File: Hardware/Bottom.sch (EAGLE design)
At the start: 106 parts, among them IC1 OP491SOIC_N14, IC2 74AC74D, IC3 74LVC1G17DCK, IC4 LT6231, IC5 SN74CBT3253SOIC16, Q1 DMPH6050SK3, Q2 25MHz

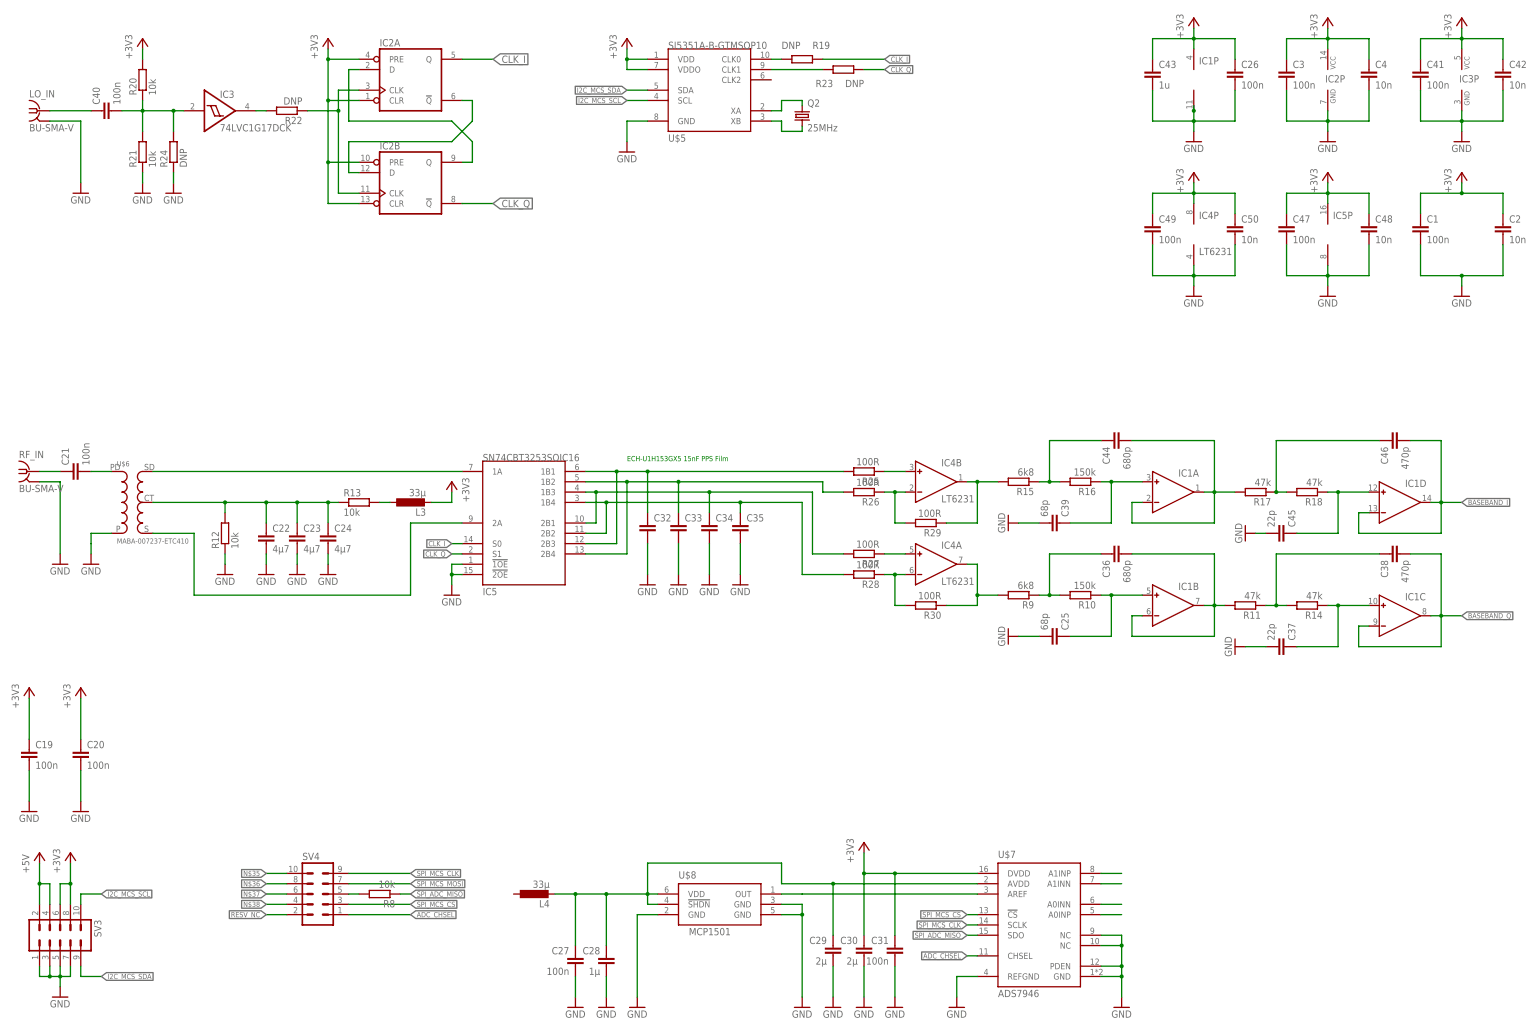
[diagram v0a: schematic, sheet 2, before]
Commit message: Add various parts
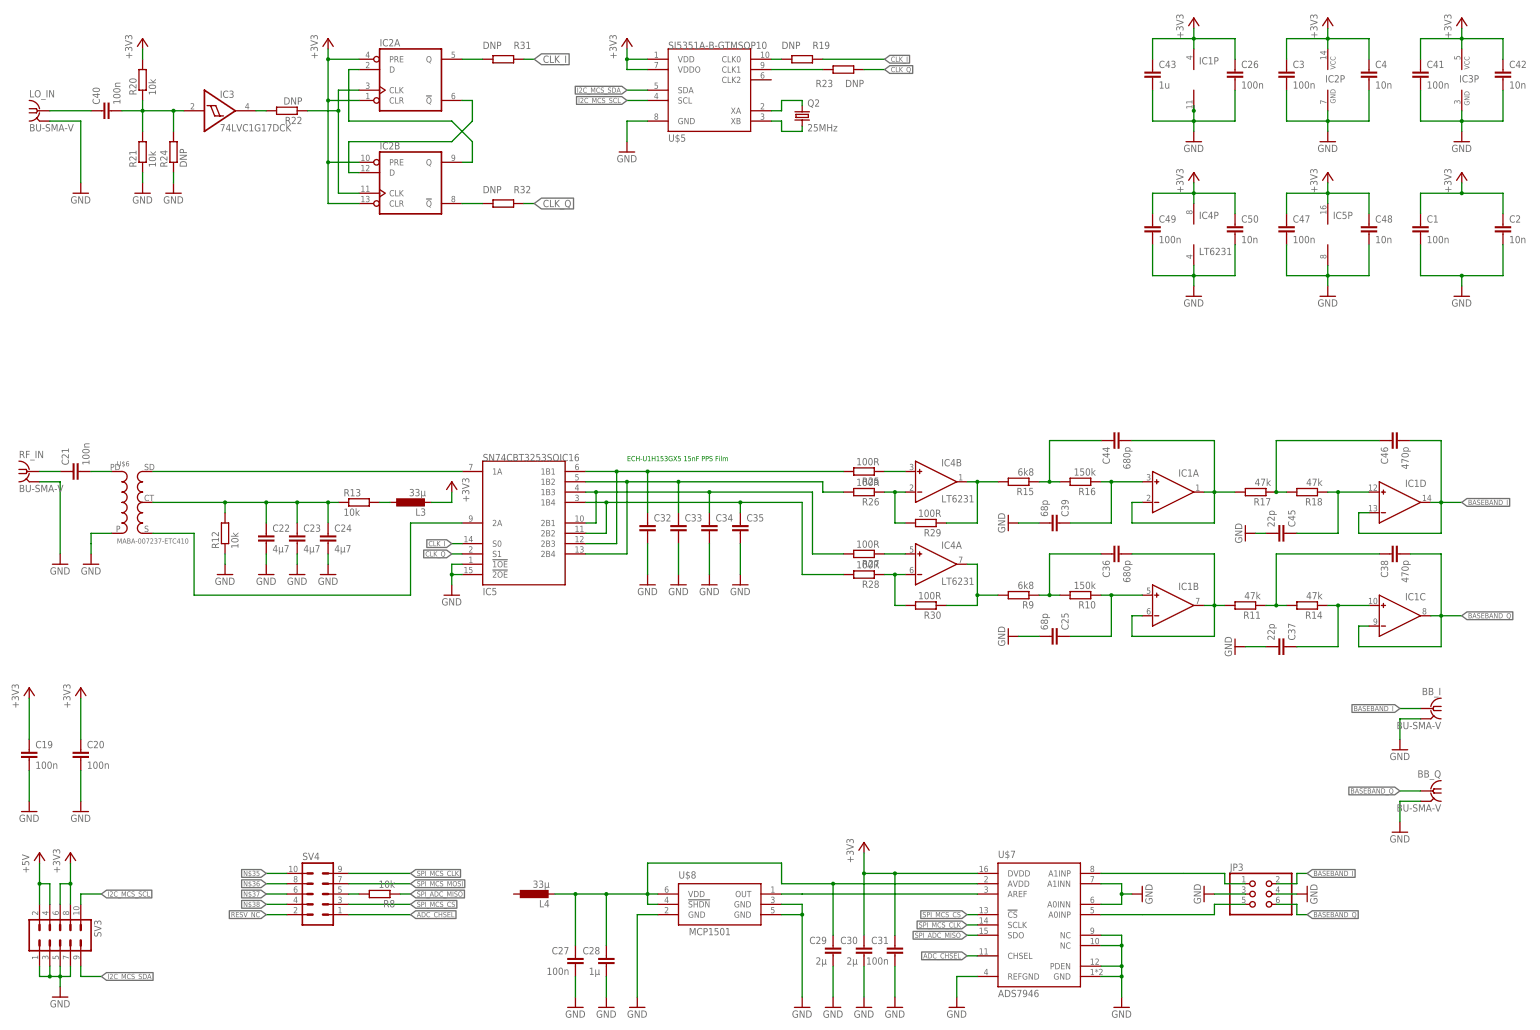
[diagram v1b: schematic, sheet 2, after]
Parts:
- added BB_I, BB_Q: BU-SMA-V, con-coax:BU-SMA-V
- added JP3: (no value), pinhead:PINHD-2X3
- added R31, R32: DNP, rcl:R-EU_R0603
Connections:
- removed net N$25: U$7.A1INP
- removed net N$28: U$7.A0INN
- new net N$58: IC2B.!Q, R32.2
- new net N$59: IC2A.Q, R31.2
- net BASEBAND_I: now also BB_I.1, JP3.2
- net BASEBAND_Q: now also BB_Q.1, JP3.6
- net CLK_I: now also R31.1; no longer IC2A.Q
- net CLK_Q: now also R32.1; no longer IC2B.!Q
- net GND: now also BB_I.2, BB_Q.2, JP3.3, JP3.4, U$7.A0INN, U$7.A1INN
- net N$26: now also JP3.1, U$7.A1INP; no longer U$7.A1INN
- net N$32: now also JP3.5

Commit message: Add various parts
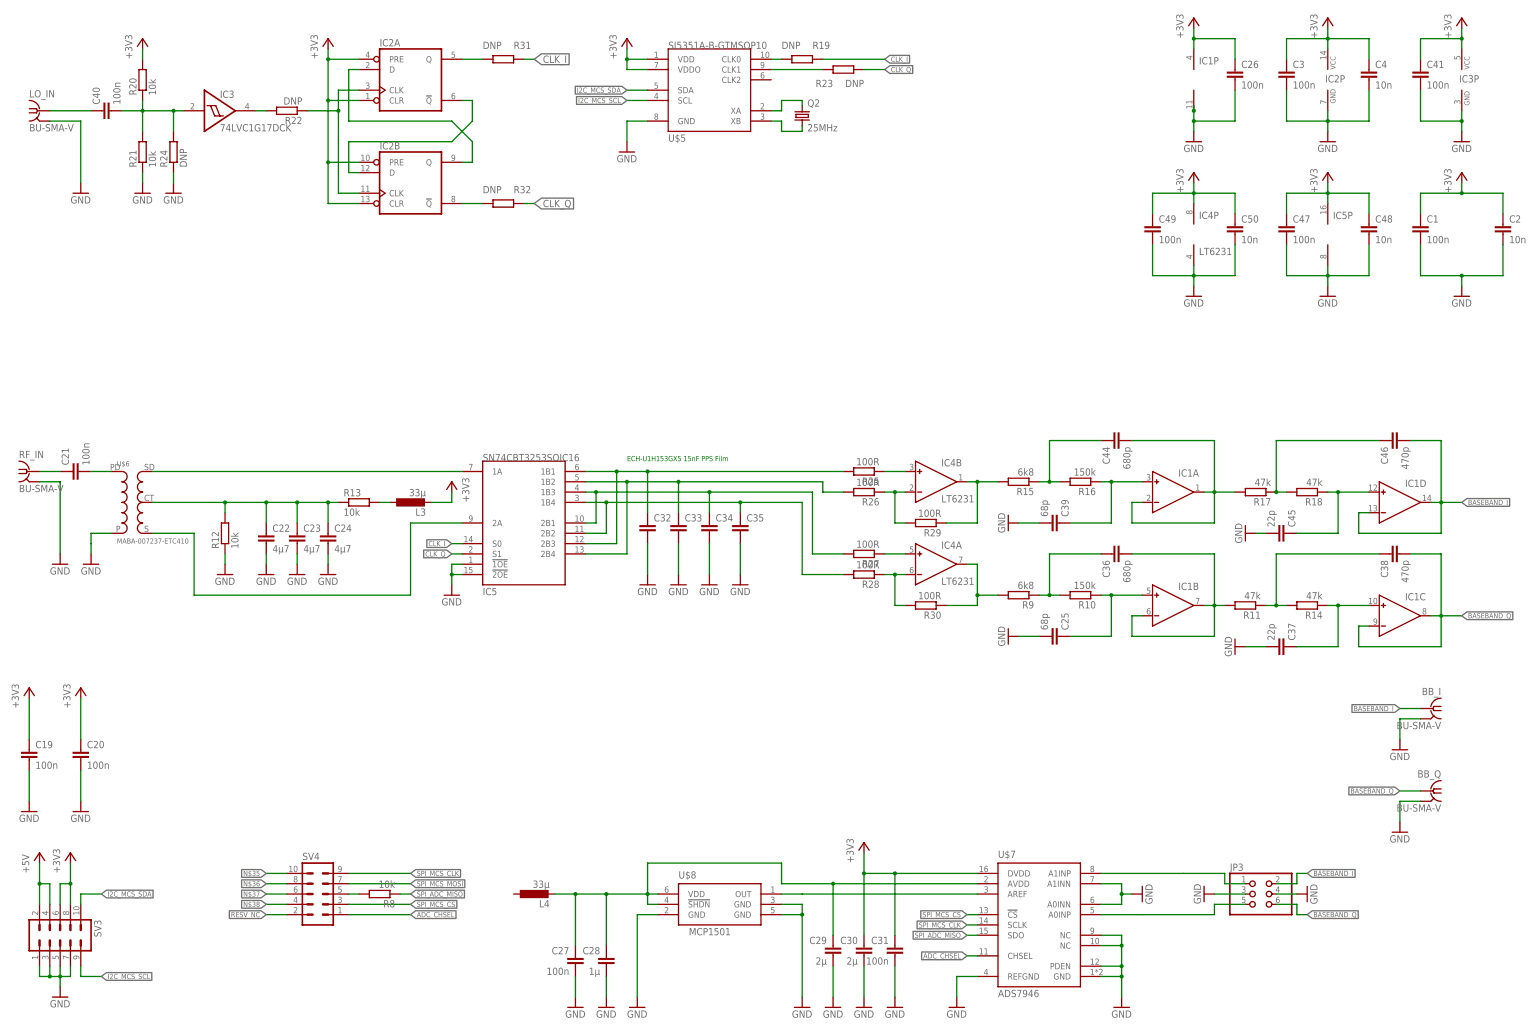
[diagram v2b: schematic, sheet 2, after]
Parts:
- removed C42: 10n, rcl:C-EUC0402
- removed C43: 1u, rcl:C-EUC0603
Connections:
- net +3V3: no longer C42.1, C43.1
- net GND: no longer C42.2, C43.2
- net I2C_MCS_SCL: now also SV3.9; no longer SV3.10
- net I2C_MCS_SDA: now also SV3.10; no longer SV3.9
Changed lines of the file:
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@@
 <part name="+3V11" library="supply1" library_urn="urn:adsk.eagle:library:371" deviceset="+3V3" device=""/>
 <part name="C41" library="rcl" library_urn="urn:adsk.eagle:library:334" deviceset="C-EU" device="C0402" package3d_urn="urn:adsk.eagle:package:23626/1" value="100n"/>
-<part name="C42" library="rcl" library_urn="urn:adsk.eagle:library:334" deviceset="C-EU" device="C0402" package3d_urn="urn:adsk.eagle:package:23626/1" value="10n"/>
 <part name="GND55" library="supply1" library_urn="urn:adsk.eagle:library:371" deviceset="GND" device=""/>
 <part name="+3V12" library="supply1" library_urn="urn:adsk.eagle:library:371" deviceset="+3V3" device=""/>
-<part name="C43" library="rcl" library_urn="urn:adsk.eagle:library:334" deviceset="C-EU" device="C0603" package3d_urn="urn:adsk.eagle:package:23616/2" value="1u"/>
 <part name="RF_IN" library="con-coax" library_urn="urn:adsk.eagle:library:133" deviceset="BU-SMA-V" device="" package3d_urn="urn:adsk.eagle:package:6211/1"/>
 <part name="LO_IN" library="con-coax" library_urn="urn:adsk.eagle:library:133" deviceset="BU-SMA-V" device="" package3d_urn="urn:adsk.eagle:package:6211/1"/>
@@
 <attribute name="VALUE" x="359.664" y="236.601" size="1.778" layer="96"/>
 </instance>
-<instance part="C42" gate="G$1" x="378.46" y="241.3" smashed="yes">
-<attribute name="NAME" x="379.984" y="241.681" size="1.778" layer="95"/>
-<attribute name="VALUE" x="379.984" y="236.601" size="1.778" layer="96"/>
-</instance>
 <instance part="GND55" gate="1" x="368.3" y="223.52" smashed="yes">
 <attribute name="VALUE" x="365.76" y="220.98" size="1.778" layer="96"/>
@@
 <instance part="+3V12" gate="G$1" x="368.3" y="254" smashed="yes">
 <attribute name="VALUE" x="365.76" y="248.92" size="1.778" layer="96" rot="R90"/>
-</instance>
-<instance part="C43" gate="G$1" x="292.1" y="241.3" smashed="yes">
-<attribute name="NAME" x="293.624" y="241.681" size="1.778" layer="95"/>
-<attribute name="VALUE" x="293.624" y="236.601" size="1.778" layer="96"/>
 </instance>
 <instance part="RF_IN" gate="G$1" x="15.24" y="142.24" smashed="yes">
@@
 <wire x1="312.42" y1="228.6" x2="302.26" y2="228.6" width="0.1524" layer="91"/>
 <junction x="302.26" y="228.6"/>
-<pinref part="C43" gate="G$1" pin="2"/>
-<wire x1="292.1" y1="236.22" x2="292.1" y2="228.6" width="0.1524" layer="91"/>
-<wire x1="292.1" y1="228.6" x2="302.26" y2="228.6" width="0.1524" layer="91"/>
 <pinref part="IC1" gate="P" pin="V-"/>
 <junction x="302.26" y="231.14"/>
@@
 <pinref part="GND55" gate="1" pin="GND"/>
 <wire x1="368.3" y1="228.6" x2="368.3" y2="226.06" width="0.1524" layer="91"/>
-<wire x1="368.3" y1="228.6" x2="378.46" y2="228.6" width="0.1524" layer="91"/>
 <junction x="368.3" y="228.6"/>
-<pinref part="C42" gate="G$1" pin="2"/>
-<wire x1="378.46" y1="228.6" x2="378.46" y2="236.22" width="0.1524" layer="91"/>
 <wire x1="368.3" y1="231.14" x2="368.3" y2="228.6" width="0.1524" layer="91"/>
 <pinref part="IC3" gate="P" pin="GND"/>
@@
 <pinref part="+3V12" gate="G$1" pin="+3V3"/>
 <wire x1="368.3" y1="248.92" x2="368.3" y2="251.46" width="0.1524" layer="91"/>
-<wire x1="368.3" y1="248.92" x2="378.46" y2="248.92" width="0.1524" layer="91"/>
 <junction x="368.3" y="248.92"/>
-<pinref part="C42" gate="G$1" pin="1"/>
-<wire x1="378.46" y1="248.92" x2="378.46" y2="243.84" width="0.1524" layer="91"/>
 <wire x1="368.3" y1="246.38" x2="368.3" y2="248.92" width="0.1524" layer="91"/>
 <pinref part="IC3" gate="P" pin="VCC"/>
@@
 <pinref part="C26" gate="G$1" pin="1"/>
 <wire x1="312.42" y1="248.92" x2="312.42" y2="243.84" width="0.1524" layer="91"/>
-<wire x1="302.26" y1="248.92" x2="292.1" y2="248.92" width="0.1524" layer="91"/>
-<pinref part="C43" gate="G$1" pin="1"/>
-<wire x1="292.1" y1="248.92" x2="292.1" y2="243.84" width="0.1524" layer="91"/>
 <pinref part="IC1" gate="P" pin="V+"/>
 <pinref part="+3V13" gate="G$1" pin="+3V3"/>
@@
 <net name="I2C_MCS_SDA" class="0">
 <segment>
+<wire x1="167.64" y1="236.22" x2="162.56" y2="236.22" width="0.1524" layer="91"/>
+<label x="162.56" y="236.22" size="1.27" layer="95" rot="R180" xref="yes"/>
+<pinref part="U$5" gate="G$1" pin="SDA"/>
+</segment>
+<segment>
+<wire x1="27.94" y1="38.1" x2="33.02" y2="38.1" width="0.1524" layer="91"/>
+<label x="33.02" y="38.1" size="1.27" layer="95" xref="yes"/>
+<pinref part="SV3" gate="G$1" pin="10"/>
+<wire x1="27.94" y1="35.56" x2="27.94" y2="38.1" width="0.1524" layer="91"/>
+</segment>
+</net>
+<net name="I2C_MCS_SCL" class="0">
+<segment>
+<wire x1="167.64" y1="233.68" x2="162.56" y2="233.68" width="0.1524" layer="91"/>
+<label x="162.56" y="233.68" size="1.27" layer="95" rot="R180" xref="yes"/>
+<pinref part="U$5" gate="G$1" pin="SCL"/>
+</segment>
+<segment>
 <wire x1="27.94" y1="17.78" x2="33.02" y2="17.78" width="0.1524" layer="91"/>
 <label x="33.02" y="17.78" size="1.27" layer="95" xref="yes"/>
@@
 <wire x1="27.94" y1="20.32" x2="27.94" y2="17.78" width="0.1524" layer="91"/>
 </segment>
-<segment>
-<wire x1="167.64" y1="236.22" x2="162.56" y2="236.22" width="0.1524" layer="91"/>
-<label x="162.56" y="236.22" size="1.27" layer="95" rot="R180" xref="yes"/>
-<pinref part="U$5" gate="G$1" pin="SDA"/>
-</segment>
-</net>
-<net name="I2C_MCS_SCL" class="0">
-<segment>
-<wire x1="27.94" y1="38.1" x2="33.02" y2="38.1" width="0.1524" layer="91"/>
-<label x="33.02" y="38.1" size="1.27" layer="95" xref="yes"/>
-<pinref part="SV3" gate="G$1" pin="10"/>
-<wire x1="27.94" y1="35.56" x2="27.94" y2="38.1" width="0.1524" layer="91"/>
-</segment>
-<segment>
-<wire x1="167.64" y1="233.68" x2="162.56" y2="233.68" width="0.1524" layer="91"/>
-<label x="162.56" y="233.68" size="1.27" layer="95" rot="R180" xref="yes"/>
-<pinref part="U$5" gate="G$1" pin="SCL"/>
-</segment>
-</net>
+</net>
